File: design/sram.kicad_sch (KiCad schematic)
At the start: 43 parts, among them U11 IS61WV12816EDBLL-10TLI

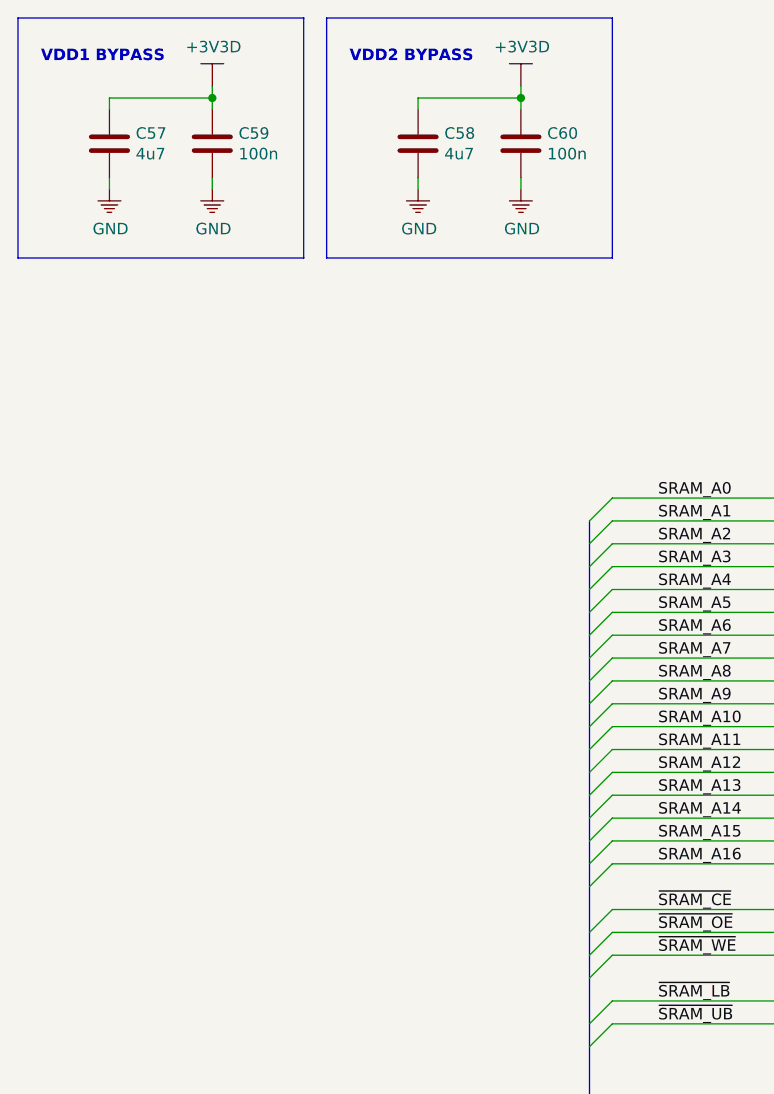
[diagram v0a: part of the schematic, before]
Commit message: Updated LNA
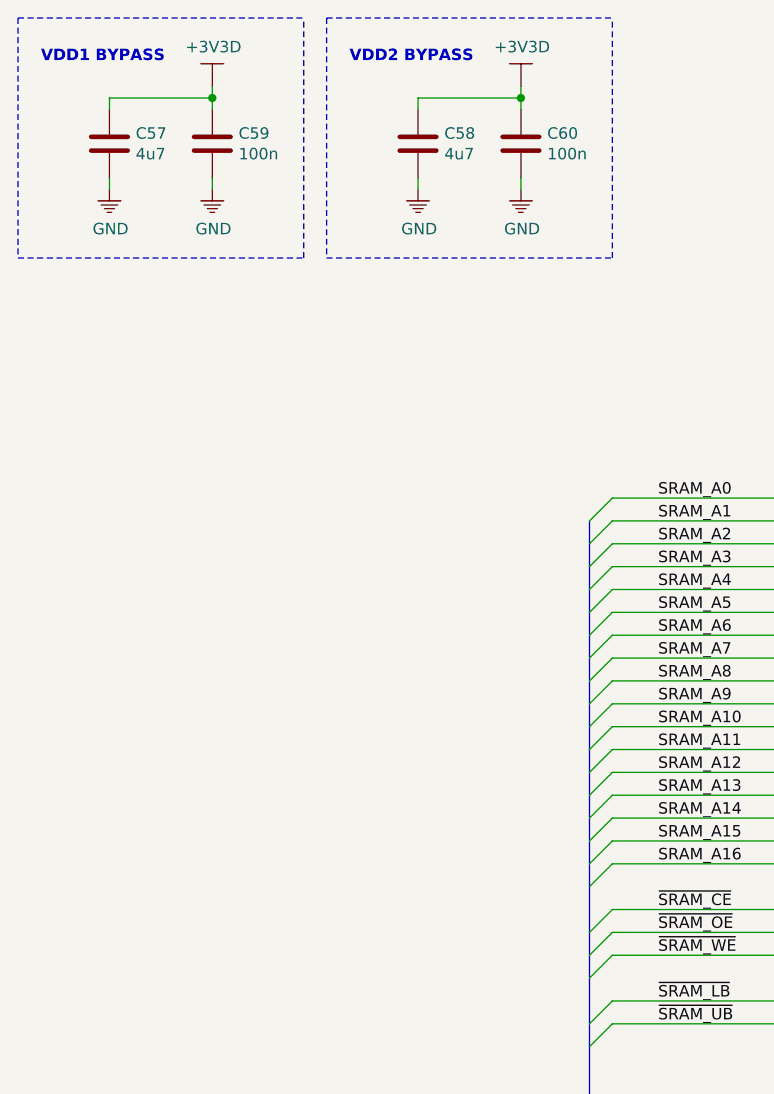
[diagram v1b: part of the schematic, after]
